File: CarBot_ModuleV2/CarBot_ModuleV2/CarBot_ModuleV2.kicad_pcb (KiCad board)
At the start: 2 copper layers, 150.7 x 62 mm, 61 parts, among them J1 Line_Tracking, J10 Motor_A, J11 Motor_B, J12 RGB_LED, J2 Buck, J3 OLED, J4 Line_Tracking, J5 Batt_1, J6 Batt_2, J7 Barrel_Jack_Switch, J8 Ultrasonic, J9 TFT_Display, Q1 SS8050, Q2 AO3401A, SW1 B1, U1 TCRT5000_C, U2 TCRT5000_L, U3 TCRT5000_R, U8 AMS1117-3.3

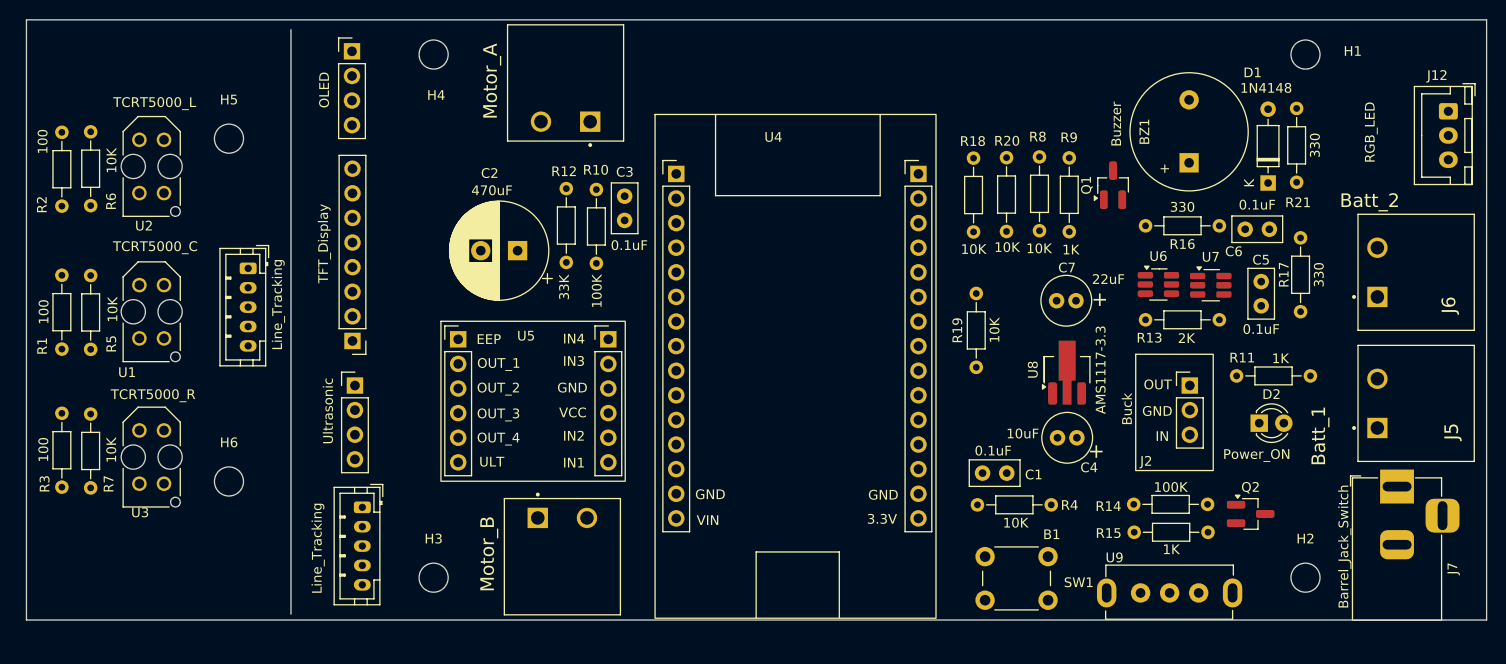
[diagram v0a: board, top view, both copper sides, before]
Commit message: Finsh car module V2
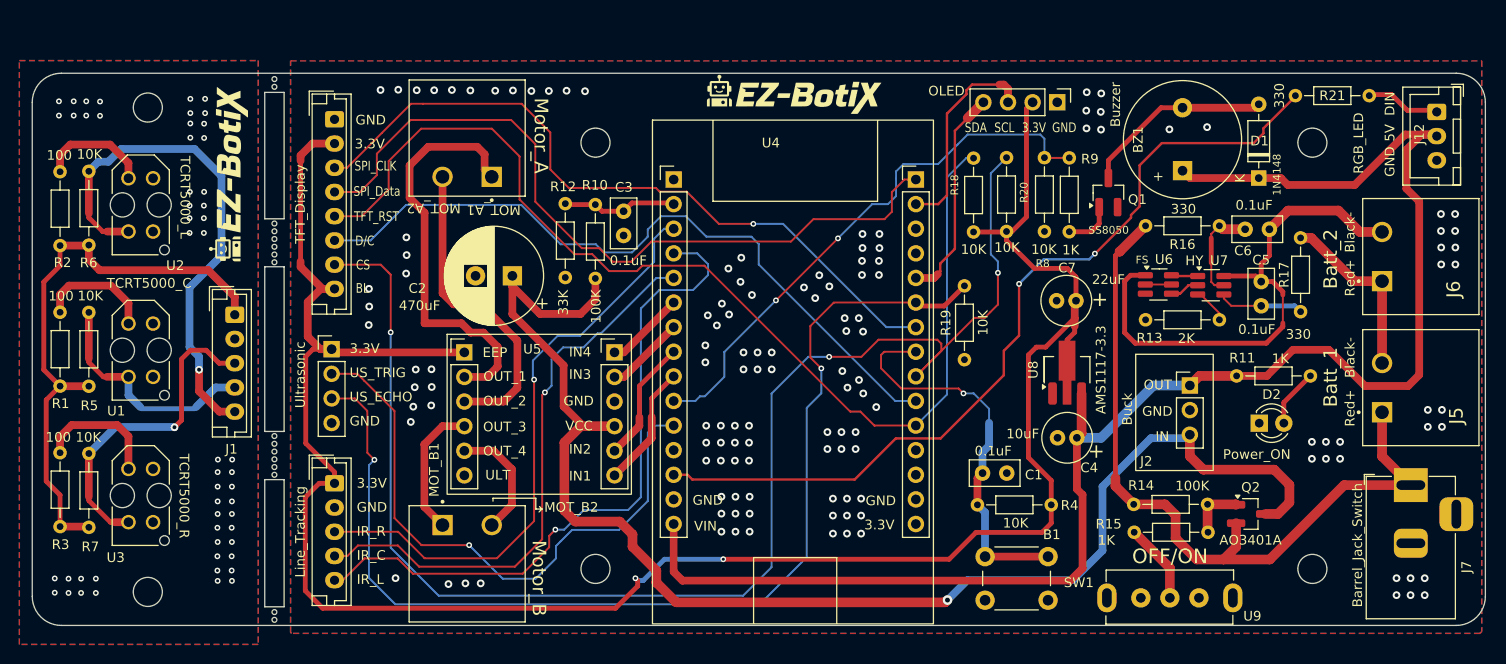
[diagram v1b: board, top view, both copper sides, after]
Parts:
- added G***: LOGO, CarBotLibrary:EZ-BotixLogoTxt, F.Cu at (154.5, 41.3)
- added G***: LOGO, CarBotLibrary:EZ-BotixLogoTxt, F.Cu at (97.2, 48.6)
- added G***: LOGO, CarBotLibrary:EZ-BotixLogo_Background, B.Cu at (153.9, 68.0)
- added G***: LOGO, CarBotLibrary:EZ-BotixLogoTxt, B.Cu at (171.0, 67.6)
- J1, J4: footprint Connector_JST:JST_PH_B5B-PH-K_1x05_P2.00mm_Vertical -> Connector_JST:JST_EH_B5B-EH-A_1x05_P2.50mm_Vertical
- J9: footprint Connector_PinHeader_2.54mm:PinHeader_1x08_P2.54mm_Vertical -> Connector_JST:JST_EH_B8B-EH-A_1x08_P2.50mm_Vertical
- moved J3 73.0 mm to (181.7, 41.1), turned to -90 degrees
- moved J9 23.0 mm to (107.1, 42.9), turned to -90 degrees
- moved H4 19.0 mm to (134.1, 45.3)
- moved H3 16.7 mm to (134.1, 89.3)
- moved H6 14.1 mm to (87.8, 91.6)
- moved J10 11.6 mm to (123.3, 48.8)
- moved J11 9.86 mm to (118.3, 84.7)
- moved H1 9.12 mm to (208.1, 45.3)
- moved H5 8.97 mm to (87.8, 41.6)
- moved R21 8.94 mm to (206.3, 40.4), turned to 0 degrees
- moved J1 4.98 mm to (96.8, 63.0)
- moved J8 4.46 mm to (106.8, 66.6)
- moved U1 4.13 mm to (87.1, 66.7)
- moved U2 4.13 mm to (87.1, 51.7)
- moved U3 4.13 mm to (87.1, 81.7)
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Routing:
- net /3.3V: track 0.00 -> 221.6 mm, vias 0 -> 2
- net /5V: track 0.00 -> 164.1 mm
- net /V_SYS: track 0.00 -> 147.8 mm, vias 0 -> 1
- net /CS: track 0.00 -> 147.1 mm, vias 0 -> 3
- net /US_ECHO: track 0.00 -> 113.2 mm, vias 0 -> 2
- net /TFT_RST: track 0.00 -> 111.7 mm
- net /RGB_EN: track 0.00 -> 88.4 mm, vias 0 -> 2
- net /B+: track 0.00 -> 79.6 mm
- net /SPI_DATA: track 0.00 -> 78.6 mm
- net /D/C: track 0.00 -> 74.7 mm
- net /SPI_CLK: track 0.00 -> 74.5 mm, vias 0 -> 1
- net /IR_S_L: track 0.00 -> 70.1 mm, vias 0 -> 1
- net /US_TRIG: track 0.00 -> 62.0 mm, vias 0 -> 1
- net /IR_S_R: track 0.00 -> 61.5 mm, vias 0 -> 1
- net /3.3V_S: track 0.00 -> 60.6 mm
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- added copper zone on B.Cu, net /GND
- added copper zone on F.Cu, net /GND
- added copper zone on B.Cu, net /GND_S
- added copper zone on F.Cu, net /GND_S
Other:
- board size 150.7 x 62 mm -> 150 x 57 mm
- board text added: "3.3V"
- board text added: "5V"
- board text added: "BL"
- board text added: "Black-"
- board text added: "CS"
- board text added: "D/C"
- board text added: "DIN"
- board text added: "FS"
- board text added: "GND"
- board text added: "HY"
- board text added: "IR_C"
- board text added: "IR_L"
- board text added: "IR_R"
- board text added: "MOT_A1"
- board text added: "MOT_A2"
- board text added: "MOT_B1"
- board text added: "MOT_B2"
- board text added: "OFF/ON"
- board text added: "Red+"
- board text added: "SCL"
- board text added: "SDA"
- board text added: "SPI_CLK"
- board text added: "SPI_Data"
- board text added: "TFT_RST"
- board text added: "US_ECHO"
- board text added: "US_TRIG"
